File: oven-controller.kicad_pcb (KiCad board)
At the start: 2 copper layers, 48.3 x 38.1 mm, 20 parts, among them J1 USB, J2 ISP, J3 Thermocouple, J4 Load In, J5 Neut In, U1 ATMEGA16U2, U2 MAX31855KASA, U3 MOC3022S, U4 LTV-354T, Y1 16MHz

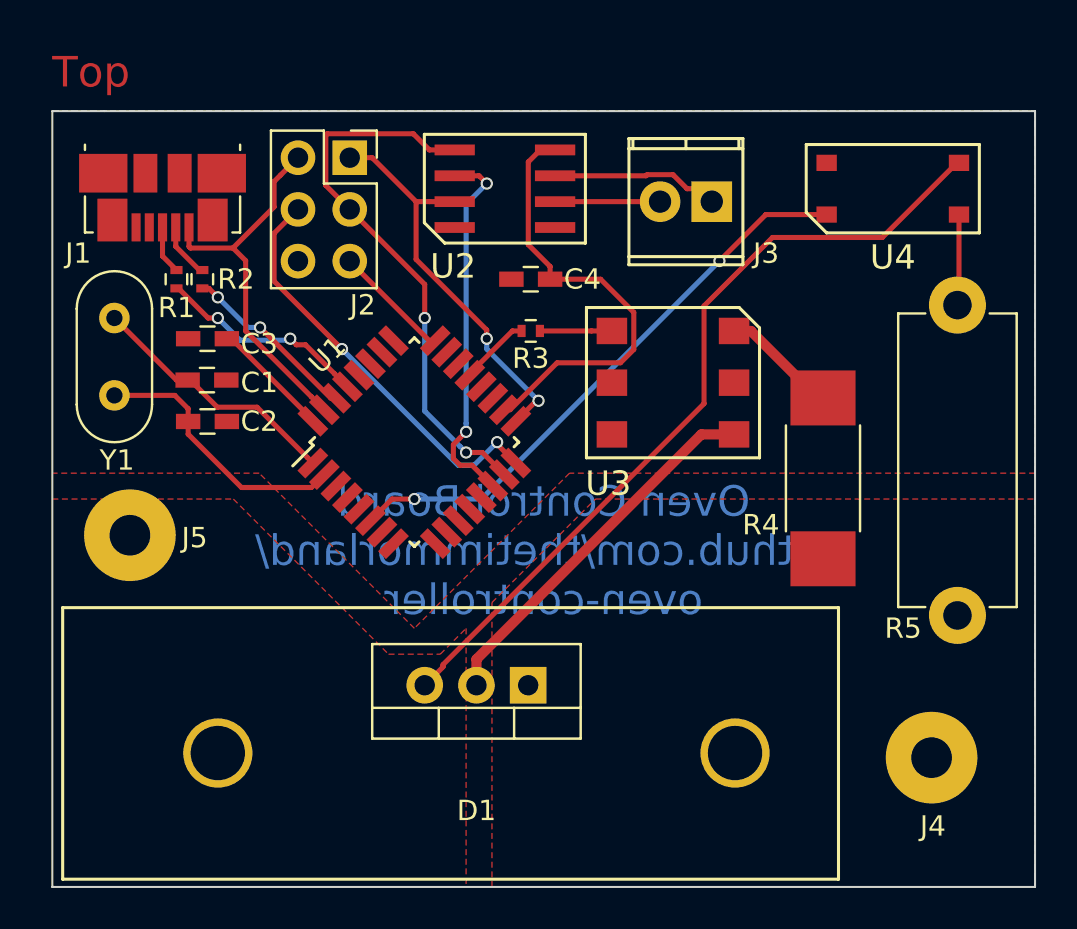
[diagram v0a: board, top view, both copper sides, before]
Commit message: oven-controller v2
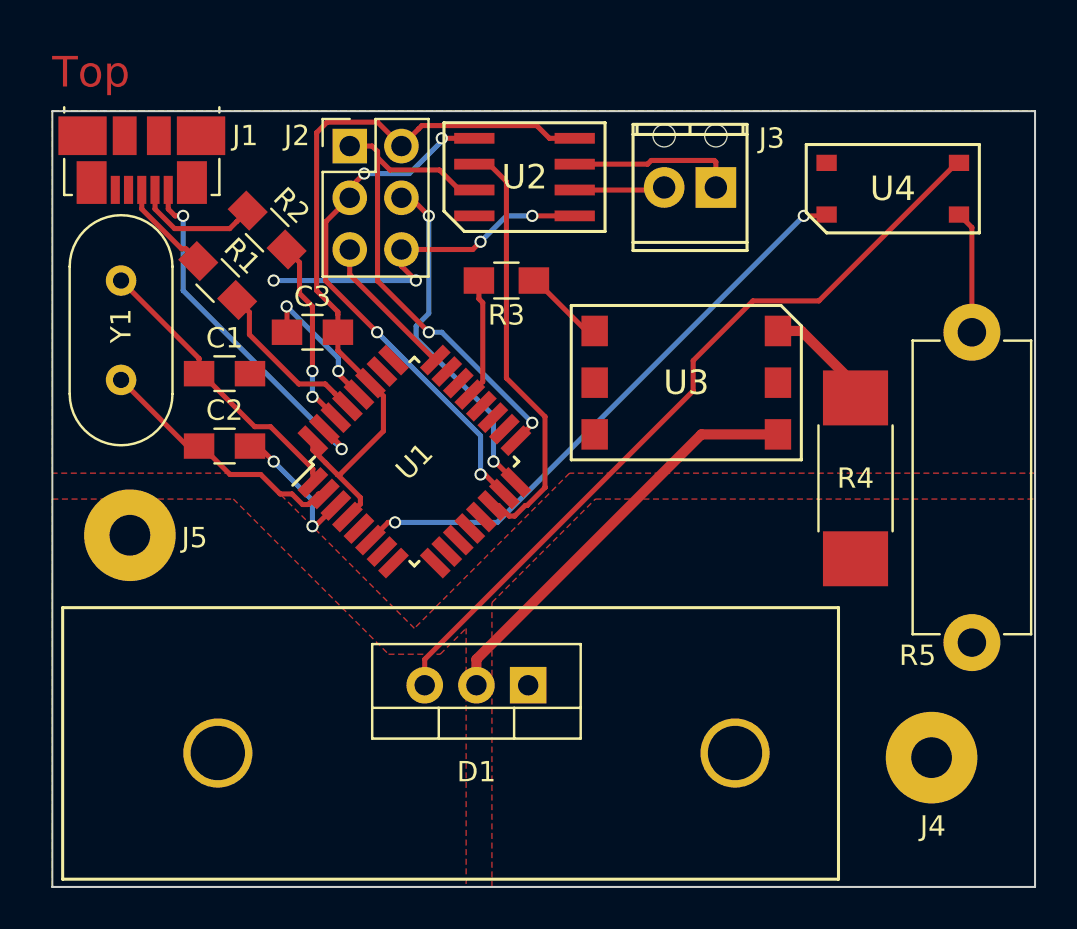
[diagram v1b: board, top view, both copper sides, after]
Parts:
- removed C4: 0.1uF, Capacitors_SMD:C_0603_HandSoldering
- C1, C2, C3: footprint Capacitors_SMD:C_0603_HandSoldering -> Capacitors_SMD:C_0805_HandSoldering
- J2: footprint Socket_Strips:Socket_Strip_Straight_2x03_Pitch2.54mm -> Pin_Headers:Pin_Header_Straight_2x03_Pitch2.54mm
- J3: footprint TerminalBlock_Phoenix_MPT-2.54mm_2pol -> TerminalBlocks_Phoenix:TerminalBlock_Phoenix_MPT-2.54mm_2pol
- R1, R2, R3: footprint Resistors_SMD:R_0402 -> Resistors_SMD:R_0805_HandSoldering
- Y1: footprint Crystals:Crystal_HC52-U_Vertical -> Crystals:Crystal_HC49-U_Vertical
- moved C3 5.16 mm to (135.9, 88.9)
- moved R2 4.00 mm to (133.7, 83.9), turned to 135 degrees
- moved R3 2.75 mm to (145.4, 86.4)
- moved J1 2.10 mm to (127.5, 79.2)
- moved R1 2.03 mm to (131.2, 86.4), turned to 135 degrees
- moved Y1 1.87 mm to (126.5, 86.4)
- moved R4 1.60 mm to (162.6, 96.1)
- moved R5 1.51 mm to (168.3, 104.1)
- moved C2 1.47 mm to (131.6, 94.5)
- moved U2 1.12 mm to (146.3, 81.3)
- moved U1 0.95 mm to (140.9, 95.2)
- moved C1 0.92 mm to (131.6, 90.9)
- moved J3 0.73 mm to (155.7, 81.8)
- moved U3 0.65 mm to (154.2, 91.4)
- moved J2 0.57 mm to (137.7, 79.8)
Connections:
- C3 pad 2: Net-(C3-Pad2) -> +3V3
- J1 pad 1: VBUS -> Net-(J1-Pad1)
- J1 pad 6: Net-(J1-Pad6) -> GND
- J2 pad 2: VBUS -> +3V3
- U1 pad 18: /3.3V -> Net-(U1-Pad18)
- U1 pad 27: Net-(C3-Pad2) -> +3V3
- U1 pad 31: VBUS -> Net-(J1-Pad1)
- U1 pad 32: Net-(C3-Pad2) -> +3V3
- U1 pad 4: Net-(C3-Pad2) -> +3V3
- U2 pad 4: /3.3V -> +3V3
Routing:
- net +3V3: track 0.00 -> 38.2 mm
- net GND: track 0.00 -> 32.1 mm, vias 0 -> 8
- net /3.3V: track 21.9 -> 0.00 mm
- net VBUS: track 18.7 -> 0.00 mm
- net Net-(J1-Pad1): track 0.00 -> 17.8 mm, vias 0 -> 2
- net Net-(C3-Pad2): track 5.94 -> 0.00 mm
- net /MISO: track 19.8 -> 25.2 mm
- net Net-(J1-Pad2): track 2.72 -> 6.26 mm
- net /MOSI: track 20.6 -> 17.1 mm
- net /SS: track 18.4 -> 21.1 mm, vias 2 -> 0
- net Net-(R3-Pad2): track 3.49 -> 5.94 mm
- net Net-(J1-Pad3): track 2.38 -> 4.77 mm
- net Net-(R1-Pad1): track 10.5 -> 8.22 mm, vias 2 -> 0
- net Net-(D1-Pad2): track 18.5 -> 20.7 mm
- net Net-(C1-Pad1): track 12.7 -> 14.3 mm
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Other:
- board text removed: "Oven Control Board github.com/thetimmorland/ oven-controller"
